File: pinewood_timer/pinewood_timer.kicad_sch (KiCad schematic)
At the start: 1 part, among them U1 STM32F091RCTx

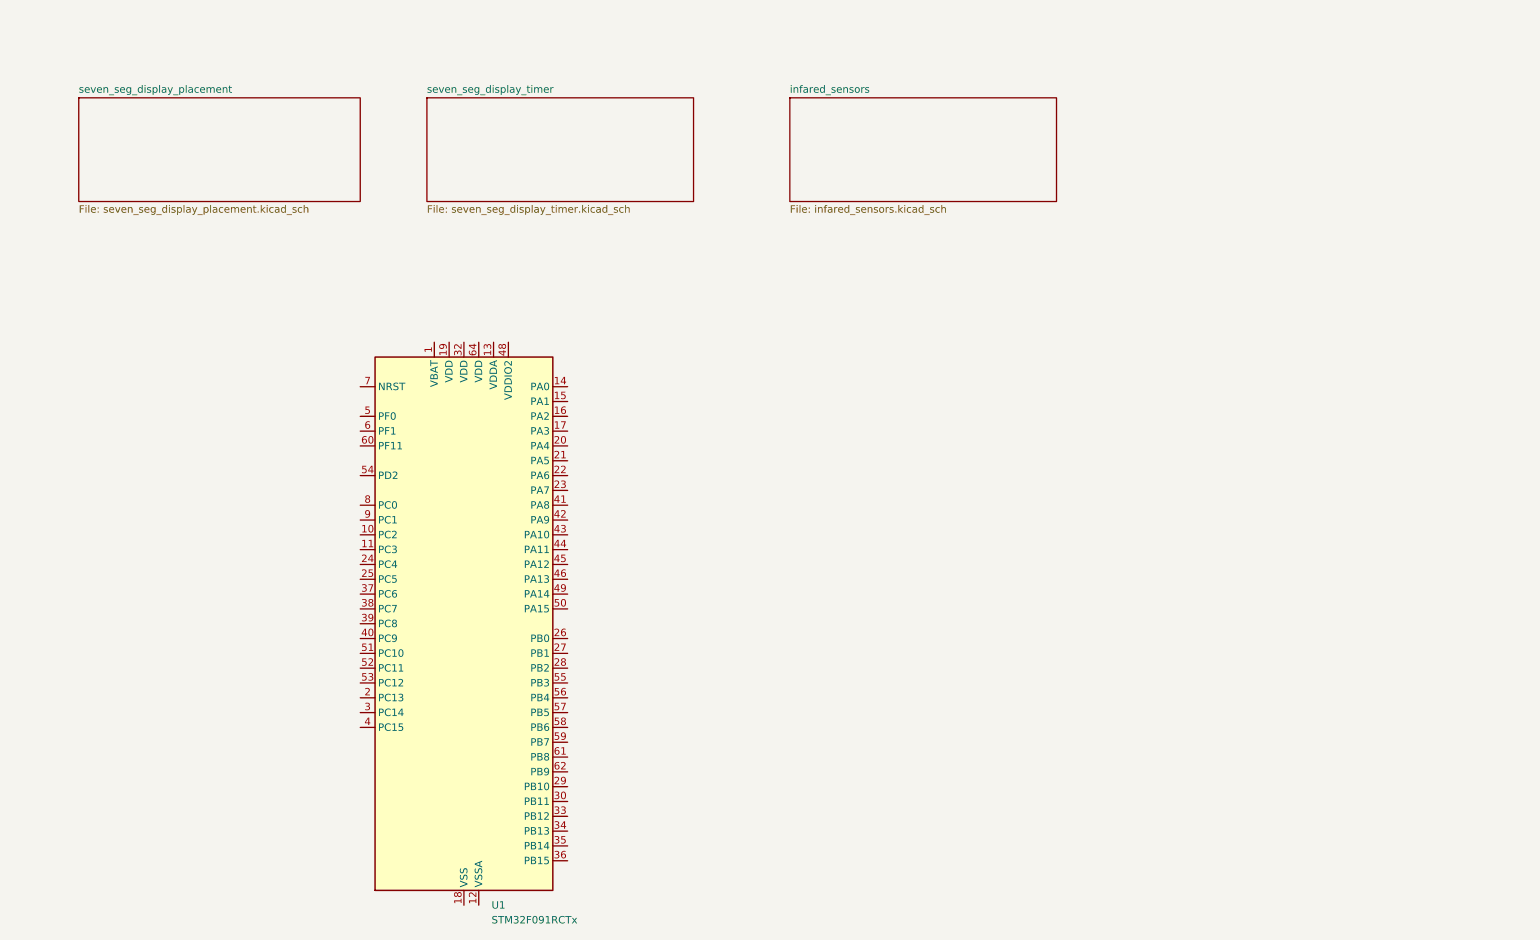
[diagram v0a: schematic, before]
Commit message: worked on schematic more
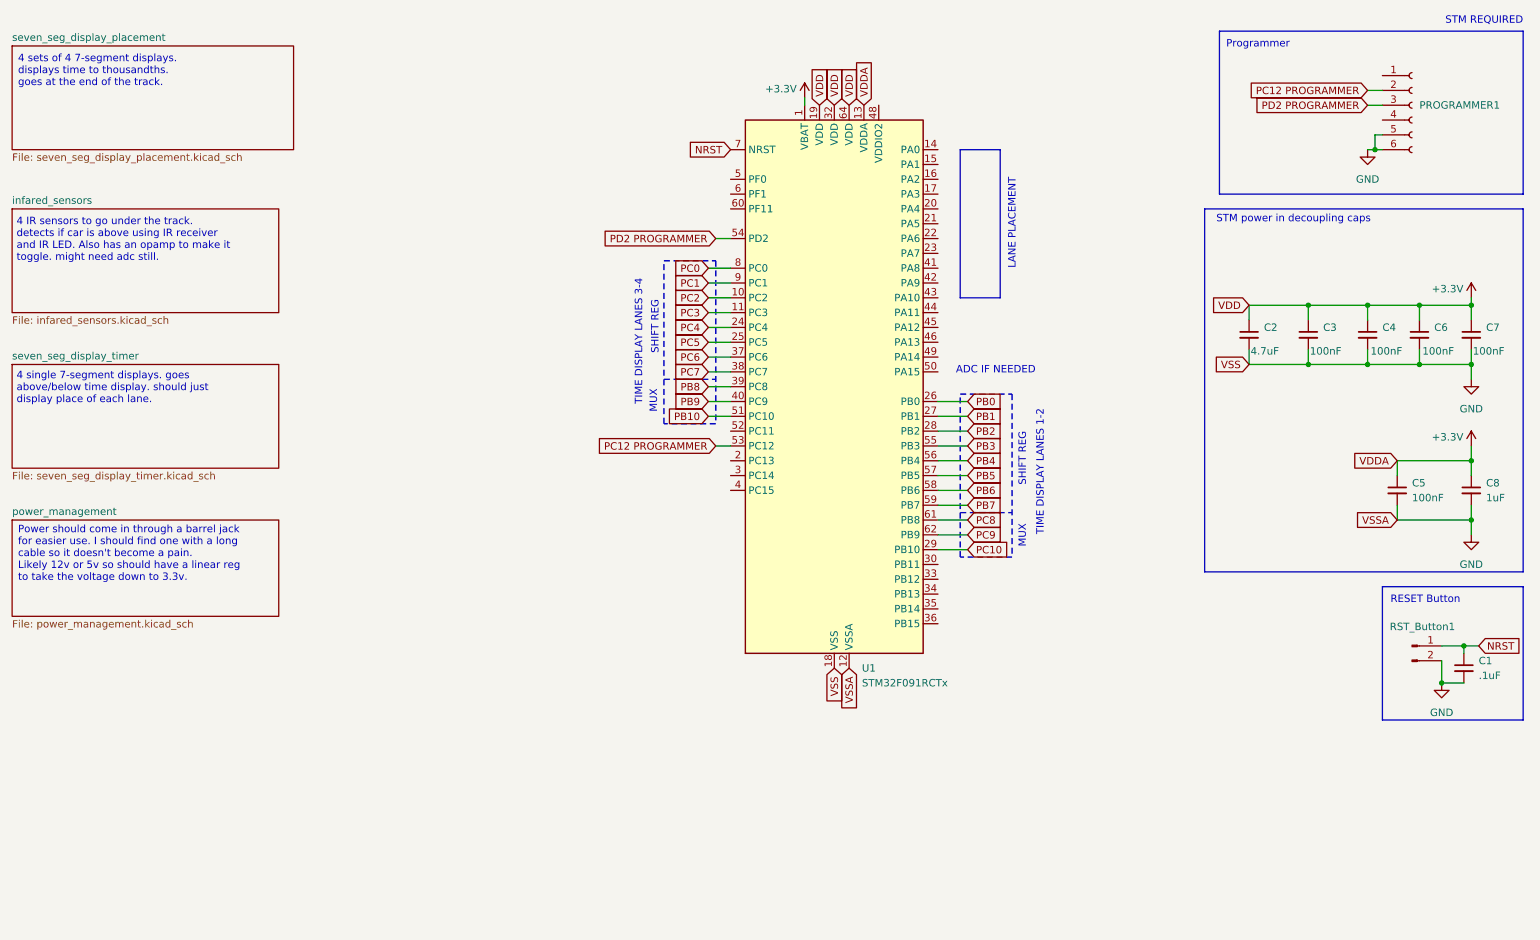
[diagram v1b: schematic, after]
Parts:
- added C1: .1uF, Capacitor_SMD:C_0805_2012Metric_Pad1.18x1.45mm_HandSolder, symbol Device:C_Small
- added C2: 4.7uF, Capacitor_SMD:C_0805_2012Metric_Pad1.18x1.45mm_HandSolder, symbol Device:C_Small
- added C3, C4, C5, C6, C7: 100nF, Capacitor_SMD:C_0805_2012Metric_Pad1.18x1.45mm_HandSolder, symbol Device:C_Small
- added C8: 1uF, Capacitor_SMD:C_0805_2012Metric_Pad1.18x1.45mm_HandSolder, symbol Device:C_Small
- added PROGRAMMER1: PROGRAMMER, Connector_PinHeader_2.54mm:PinHeader_1x06_P2.54mm_Vertical, symbol Connector:Conn_01x06_Socket
- added RST_Button1: RESET, Button_Switch_SMD:SW_SPST_CK_RS282G05A3, symbol Connector:Conn_01x02_Pin
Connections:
- net +3.3V: now reaches U1.1 (VBAT)
- net +3.3V: now also U1.13 (VDDA), U1.19 (VDD), U1.32 (VDD), U1.64 (VDD), C2.1, C3.1, C4.1, C5.1, C6.1, C7.1, C8.1
- net PC2: now reaches U1.10 (PC2)
- net PC3: now reaches U1.11 (PC3)
- net GND: now reaches U1.12 (VSSA)
- net GND: now also U1.18 (VSS), U1.31 (VSS), U1.47 (VSS), U1.63 (VSS), C1.2, C2.2, C3.2, C4.2, C5.2, C6.2, C7.2, C8.2, PROGRAMMER1.5 (Pin_5), PROGRAMMER1.6 (Pin_6), RST_Button1.2 (Pin_2)
- net PC4: now reaches U1.24 (PC4)
- net PC5: now reaches U1.25 (PC5)
- net PB0: now reaches U1.26 (PB0)
- net PB1: now reaches U1.27 (PB1)
- net PB2: now reaches U1.28 (PB2)
- net PC10: now reaches U1.29 (PB10)
- net PC6: now reaches U1.37 (PC6)
- net PC7: now reaches U1.38 (PC7)
- net PB8: now reaches U1.39 (PC8)
- net PB9: now reaches U1.40 (PC9)
- net PB10: now reaches U1.51 (PC10)
- net PC12 PROGRAMMER: now reaches U1.53 (PC12)
- net PC12 PROGRAMMER: now also PROGRAMMER1.2 (Pin_2)
- net PD2 PROGRAMMER: now reaches U1.54 (PD2)
- net PD2 PROGRAMMER: now also PROGRAMMER1.3 (Pin_3)
- net PB3: now reaches U1.55 (PB3)
- net PB4: now reaches U1.56 (PB4)
- net PB5: now reaches U1.57 (PB5)
- net PB6: now reaches U1.58 (PB6)
- net PB7: now reaches U1.59 (PB7)
- net PC8: now reaches U1.61 (PB8)
- net PC9: now reaches U1.62 (PB9)
- net NRST: now reaches U1.7 (NRST)
- net NRST: now also C1.1, RST_Button1.1 (Pin_1)
- net PC0: now reaches U1.8 (PC0)
- net PC1: now reaches U1.9 (PC1)
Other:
- added sheet power_management (power_management.kicad_sch)
- note added: "4 IR sensors to go under the track. detects if car is above using IR receiver and IR LED. Also has an opamp to make it toggle. might need adc still."
- note added: "4 sets of 4 7-segment displays. displays time to thousandths. goes at the end of the track."
- note added: "4 single 7-segment displays. goes above/below time display. should just display place of each lane."
- note added: "ADC IF NEEDED"
- note added: "LANE PLACEMENT"
- note added: "MUX"
- note added: "Power should come in through a barrel jack for easier use. I should find one with a long cable so it doesn't become a pain. Likely 12v or 5v so should have a linear reg to take the voltage down to 3.3v."
- note added: "Programmer"
- note added: "RESET Button"
- note added: "SHIFT REG"
- note added: "STM REQUIRED"
- note added: "STM power in decoupling caps"
- note added: "TIME DISPLAY LANES 1-2"
- note added: "TIME DISPLAY LANES 3-4"
- moved on the sheet: U1
